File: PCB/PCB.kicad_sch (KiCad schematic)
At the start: 0 parts

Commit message: gave up will try next time !
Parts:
- added C1: C, symbol Device:C
- added J1: USB_C_Receptacle_USB2.0_16P, symbol Connector:USB_C_Receptacle_USB2.0_16P
- added U1: STM32F407VETx, Package_QFP:LQFP-100_14x14mm_P0.5mm, symbol MCU_ST_STM32F4:STM32F407VETx
- added U2: USB3300-EZK, Package_DFN_QFN:QFN-32-1EP_5x5mm_P0.5mm_EP3.45x3.45mm, symbol Interface_USB:USB3300-EZK
- added U3: MP1584EN, MP1584EN:SOIC127P600X170-9N, symbol MP1584EN:MP1584EN
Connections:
- new net: J1.A1 (GND), J1.A12 (GND), J1.B1 (GND), J1.B12 (GND), U3.5 (GND), U3.9 (GND)
- new net: C1.1, J1.A4 (VBUS), J1.A9 (VBUS), J1.B4 (VBUS), J1.B9 (VBUS), U3.7 (VIN)
- new net: C1.2, U2.33 (GND)
- new net: U1.10 (VSS), U1.27 (VSS), U1.74 (VSS), U1.99 (VSS)

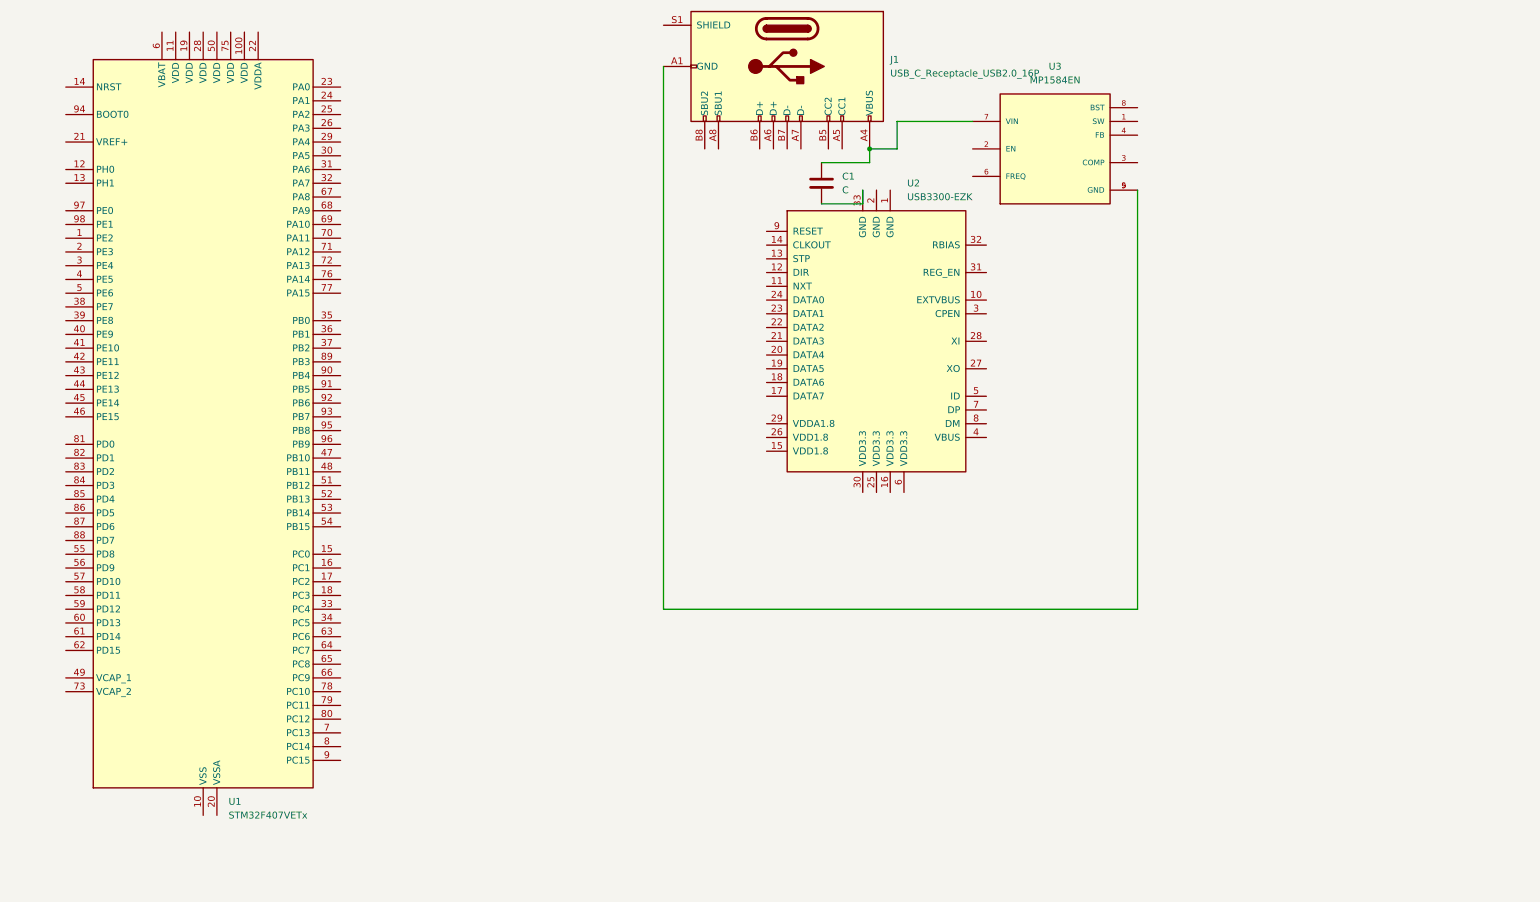
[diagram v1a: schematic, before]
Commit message: ehh
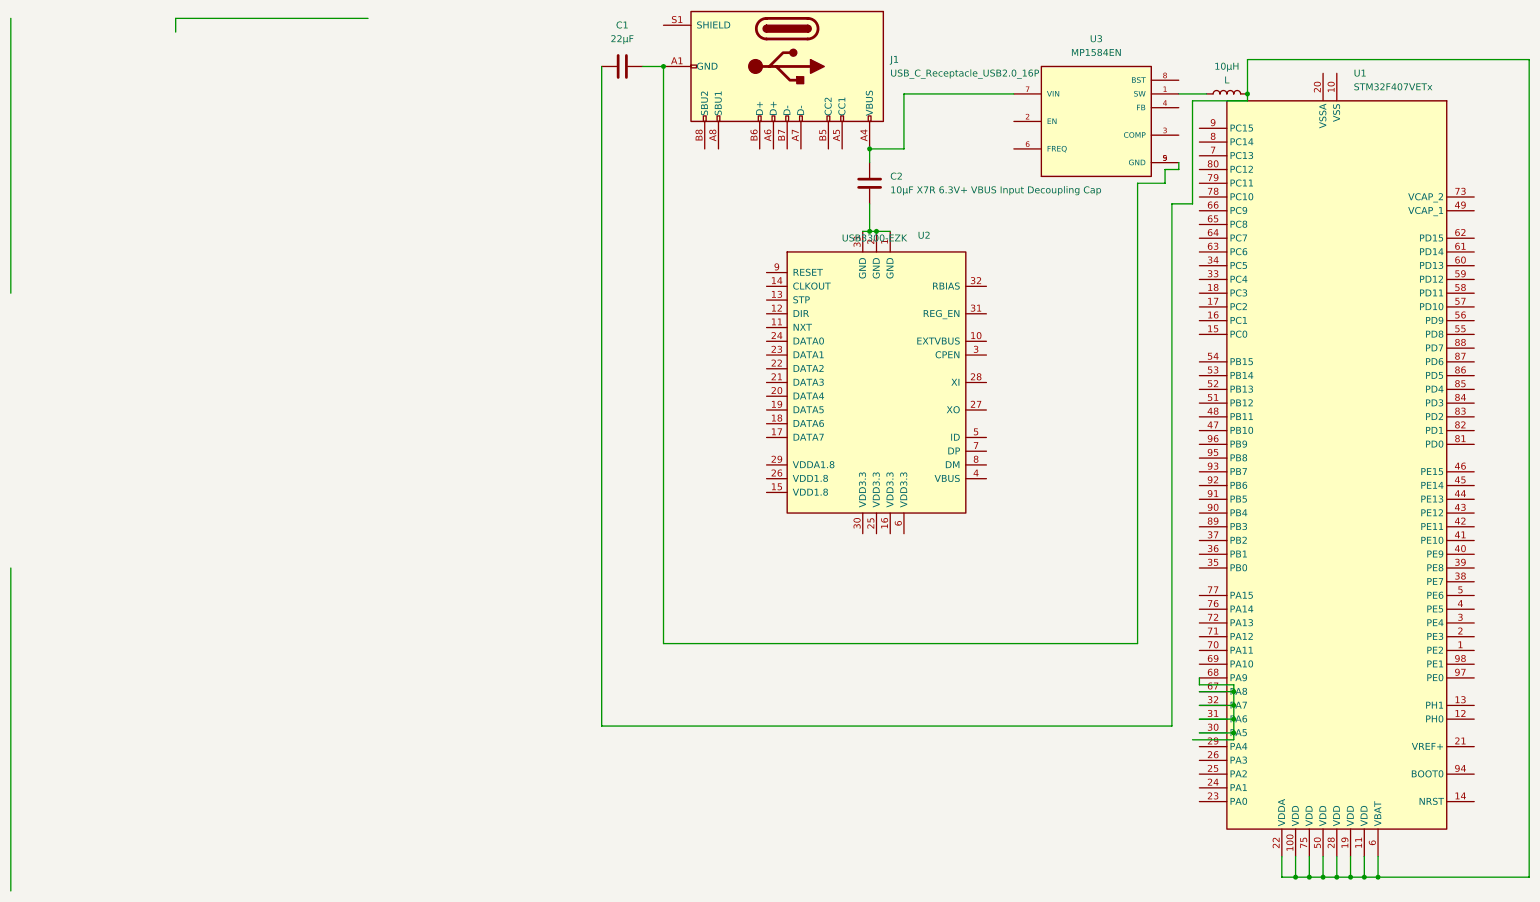
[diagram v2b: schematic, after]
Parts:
- added 10µH: L, symbol Device:L
- added C2: 10µF X7R 6.3V+ VBUS Input Decoupling Cap, symbol Device:C
- C1: value C -> 22µF
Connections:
- net at J1.A1 (GND), J1.A12 (GND), J1.B1 (GND)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: now also C1.2
- net at J1.A4 (VBUS), J1.A9 (VBUS), J1.B4 (VBUS)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: now also C2.1; no longer C1.1
- net at U2.33 (GND): now also U2.1 (GND), U2.2 (GND), C2.2; no longer C1.2
- net at U3.1 (SW): now also 10µH.1
- net at U1.100 (VDD): now also C1.1, U1.11 (VDD), U1.19 (VDD), U1.22 (VDDA), U1.28 (VDD), U1.50 (VDD), U1.6 (VBAT), U1.75 (VDD), 10µH.2
- net at U1.30 (PA5): now also U1.31 (PA6), U1.32 (PA7), U1.67 (PA8), U1.68 (PA9)
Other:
- moved on the sheet: U1, U2, U3
